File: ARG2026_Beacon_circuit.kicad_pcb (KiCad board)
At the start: 2 copper layers, 100 x 86.6 mm, 30 parts, among them J1 Conn_01x02_Pin, J2 Conn_01x02_Pin, Q1 IRLML0030, SW1 SW_SPDT, U1 CH32V002A4M6

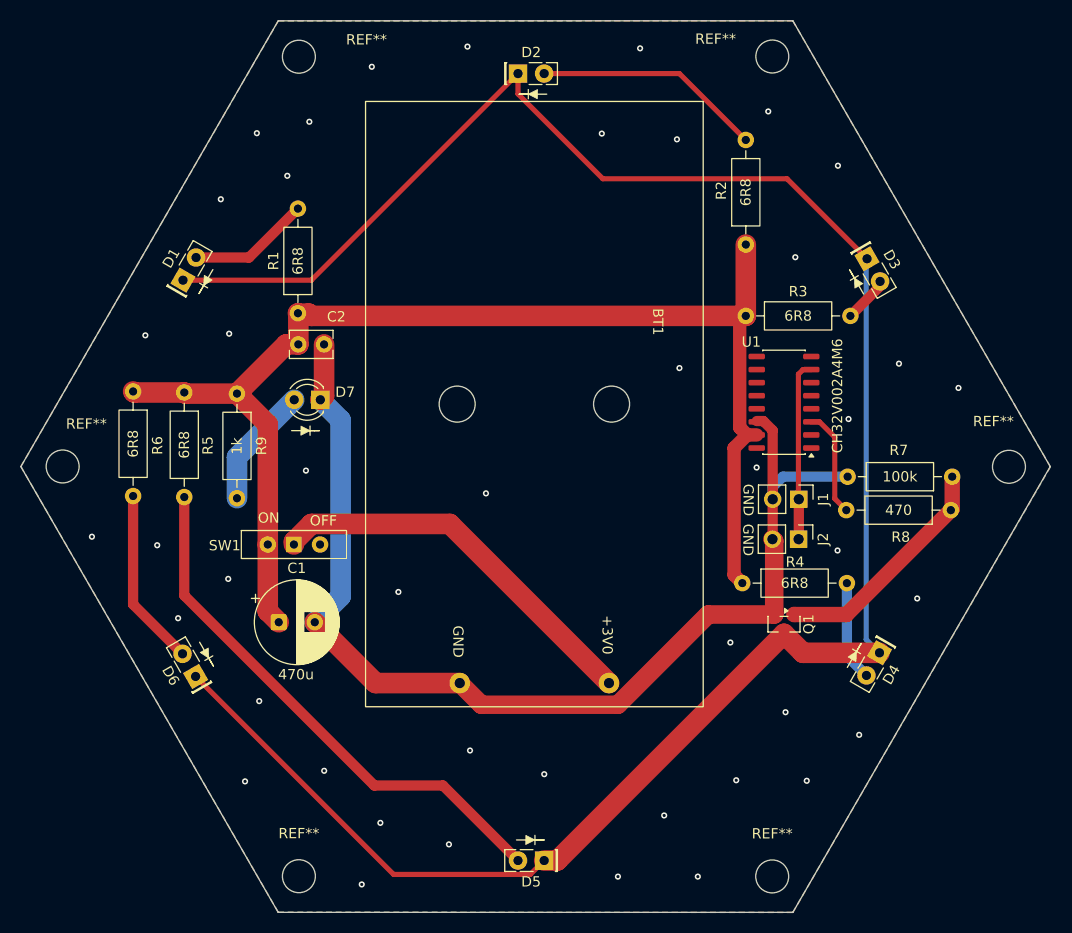
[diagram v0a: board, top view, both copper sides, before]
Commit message: feat: adjust to cnc
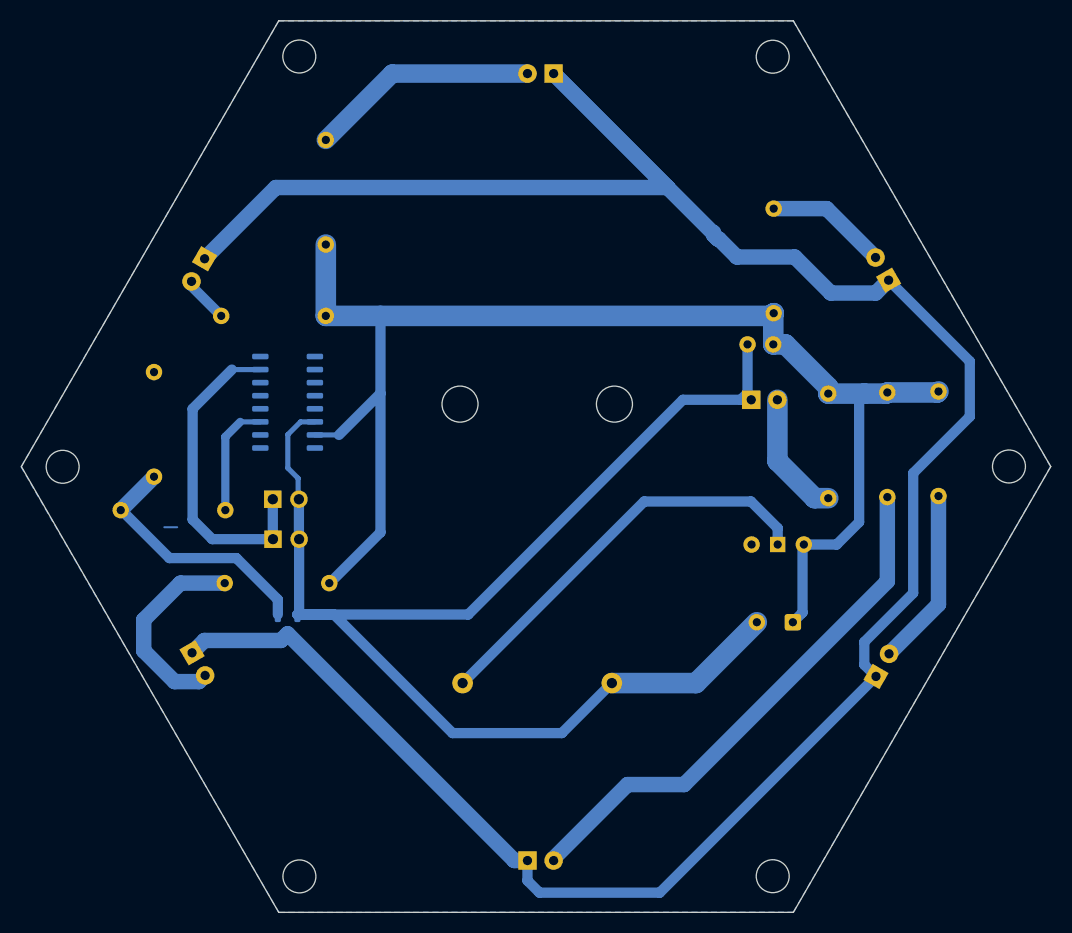
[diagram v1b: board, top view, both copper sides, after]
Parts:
- BT1, C1, C2, D1, D2, D3, D4, D5, D6, D7, J1, J2, Q1, R1, R2, R3, R4, R5, R6, R7, R8, R9, REF** (x6), SW1, U1: moved to B.Cu
- moved REF** 91.9 mm to (175.1, 101.1), turned to 180 degrees
- moved REF** 91.9 mm to (267.1, 101.1), turned to 180 degrees
- moved R8 80.6 mm to (180.8, 105.3), turned to 0 degrees
- moved R6 78.2 mm to (260.2, 93.8)
- moved R7 77.5 mm to (184.0, 102.1), turned to 90 degrees
- moved D1 68.5 mm to (255.4, 83.0), turned to 120 degrees
- moved R5 68.3 mm to (255.2, 93.9)
- moved D4 66.8 mm to (187.7, 119.2), turned to -60 degrees
- moved D6 66.1 mm to (254.1, 121.5), turned to 60 degrees
- moved D3 64.4 mm to (188.9, 80.9), turned to -120 degrees
- moved R9 57.4 mm to (249.5, 94.0)
- moved J1 51.1 mm to (195.5, 104.3)
- moved J2 51.1 mm to (195.6, 108.2)
- moved C1 49.9 mm to (246.1, 116.2), turned to 180 degrees
- moved Q1 48.2 mm to (197.0, 116.4)
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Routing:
- net Net-(D1-K): track 207.1 -> 239.5 mm
- net GND: track 109.4 -> 133.4 mm, vias 44 -> 0
- net /SWIO: track 17.5 -> 31.4 mm
- net /VDD: track 124.0 -> 135.3 mm
- net Net-(D4-A): track 9.75 -> 19.8 mm
- net Net-(BT1-+): track 38.0 -> 40.6 mm
- net Net-(Q1-G): track 22.8 -> 24.9 mm
- net (no net): track 0.00 -> 1.25 mm
- net Net-(D5-A): track 52.6 -> 52.0 mm
- net /T1C3: track 10.5 -> 11.1 mm
- net Net-(D7-A): track 11.9 -> 12.4 mm
- removed copper zone on F.Cu, net GND
